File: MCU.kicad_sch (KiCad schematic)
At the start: 82 parts, among them J401 EXPANSION, J402 RS485_1, J403 RS485_2, J404 Conn_ARM_JTAG_SWD_10, Q401 BC807, Q402 BC807, Q403 BC807, Q404 BC807, Q405 BC807, Q406 BC807, Q407 BC807, Q408 BC807, U401 TCA9535RTWR, U403 EFM32PG22C200F512IM40, U404 SN75176AD, U405 XC6204B33, Y401 Abracon_ABM11

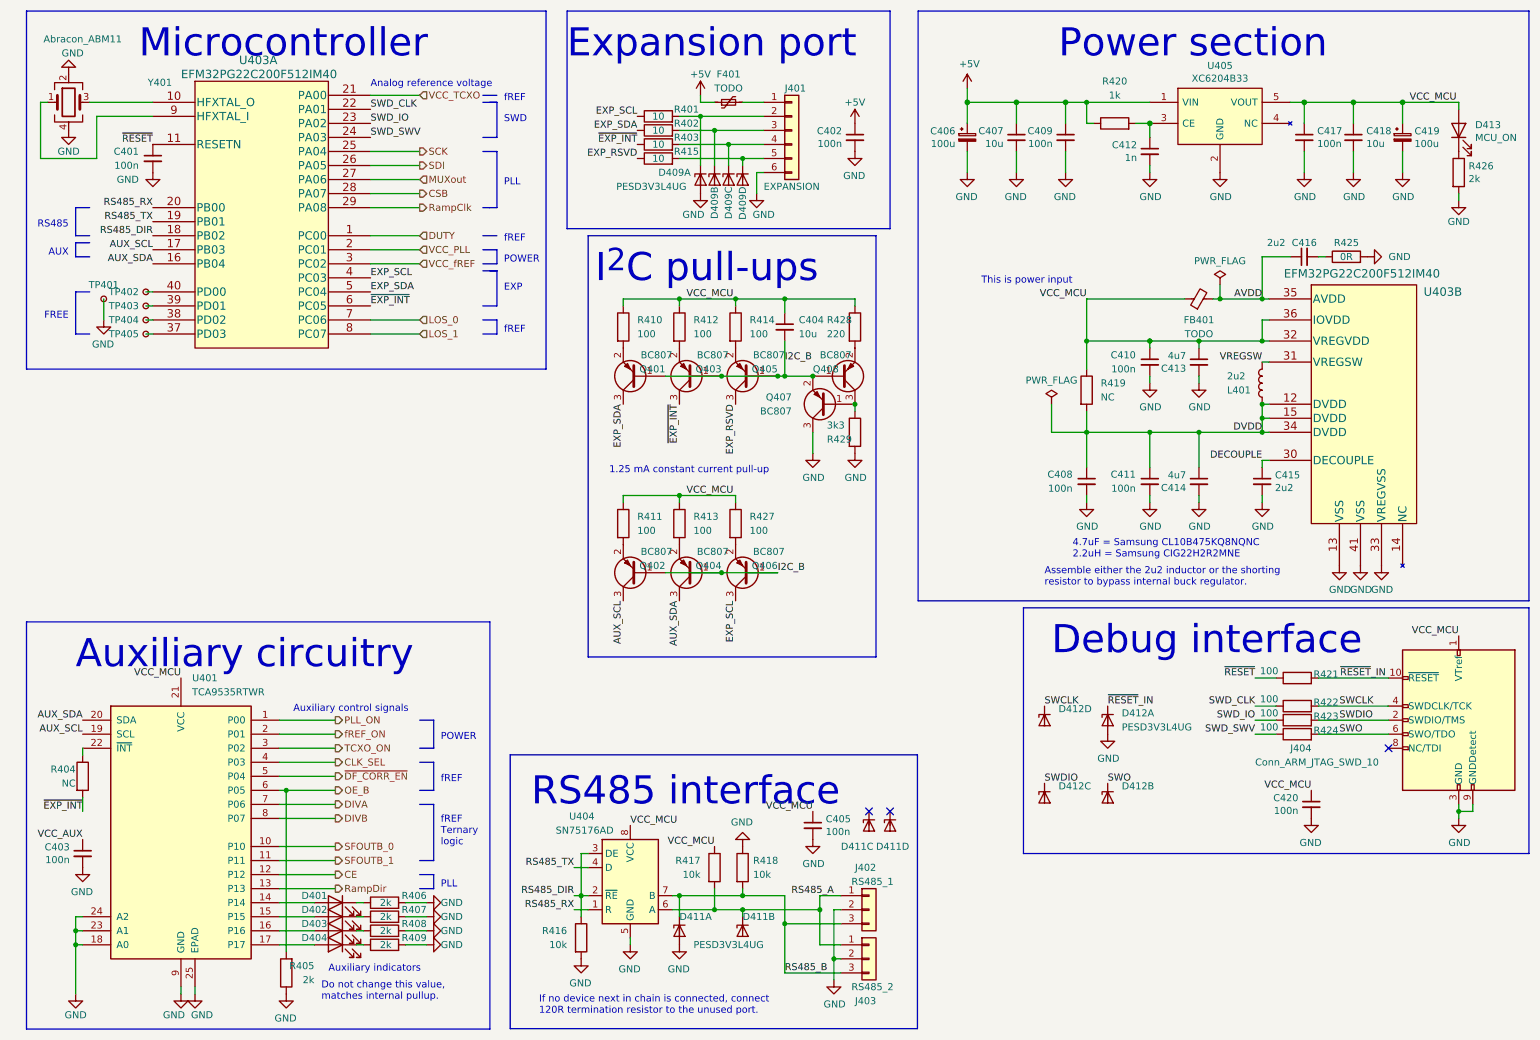
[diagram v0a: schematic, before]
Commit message: Some minor fixes
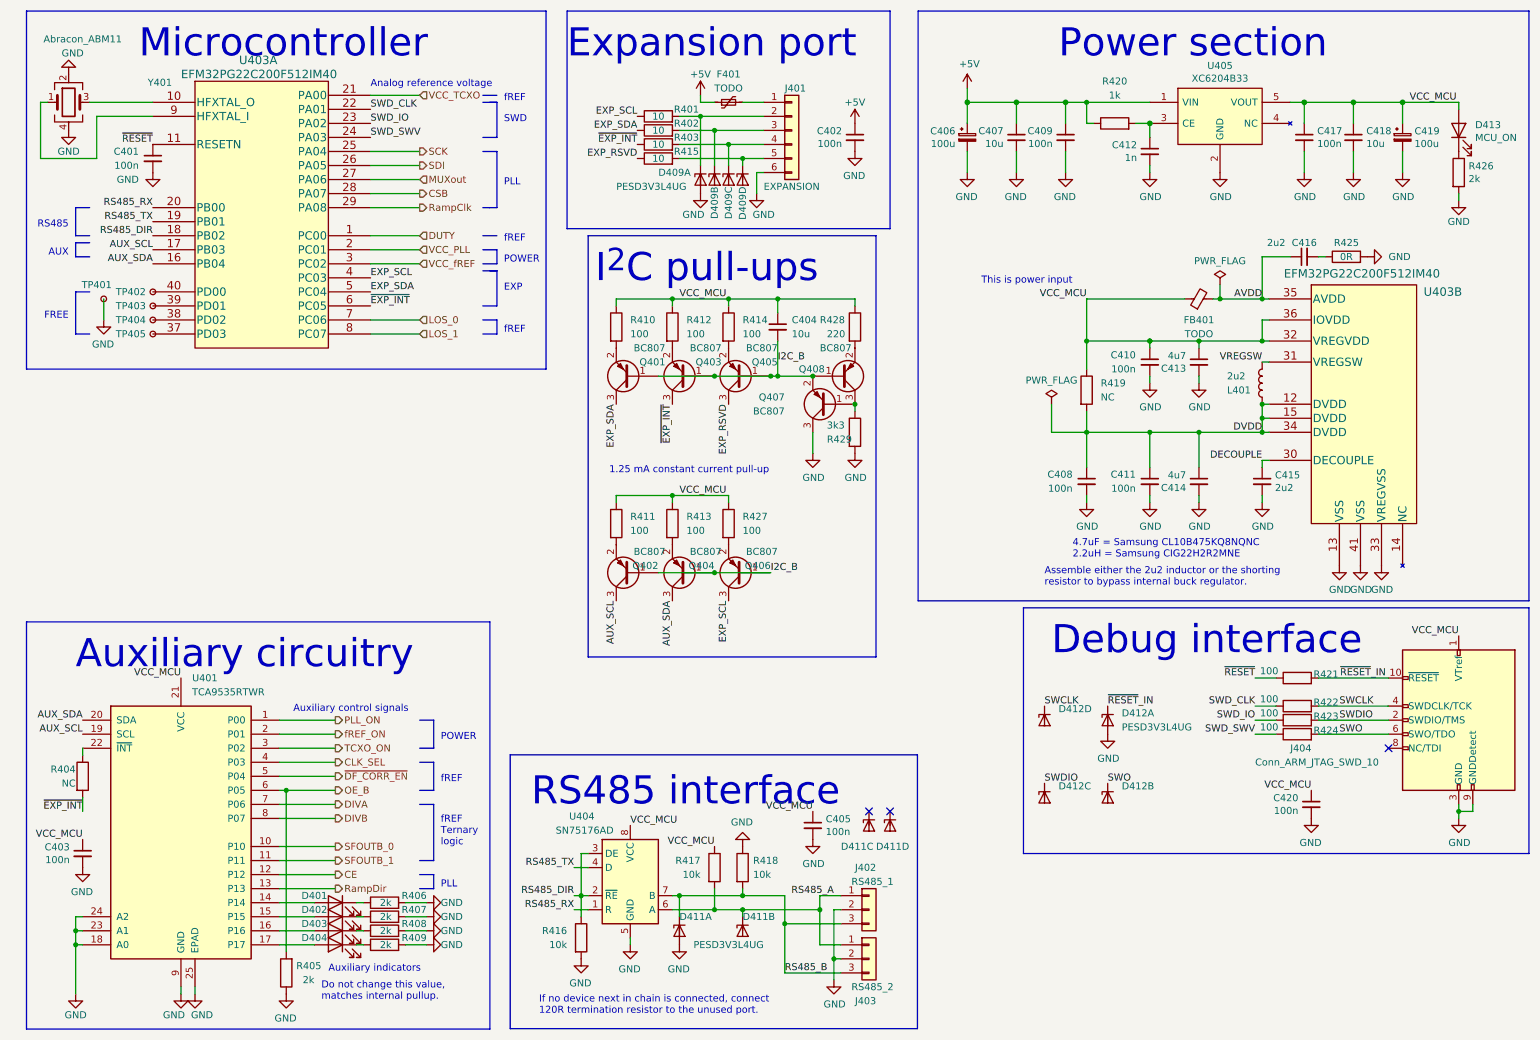
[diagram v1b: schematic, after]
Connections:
- net VCC_AUX is gone; now on net VCC_MCU: C403.1
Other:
- moved on the sheet: C404, Q401, Q402, Q403, Q404, Q405, Q406, R410, R411, R412, R413, R414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
